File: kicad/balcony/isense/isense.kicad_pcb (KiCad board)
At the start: 2 copper layers, 20.3 x 15.2 mm, 9 parts, among them J1 IN, U1 OPA237NA_250, U2 OPA237NA_250

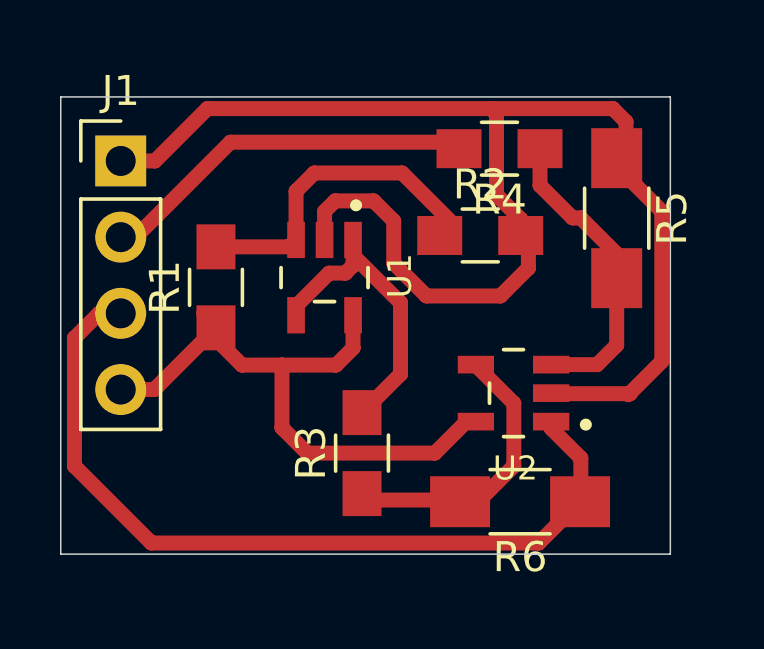
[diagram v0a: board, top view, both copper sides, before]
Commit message: Various schematic fixes
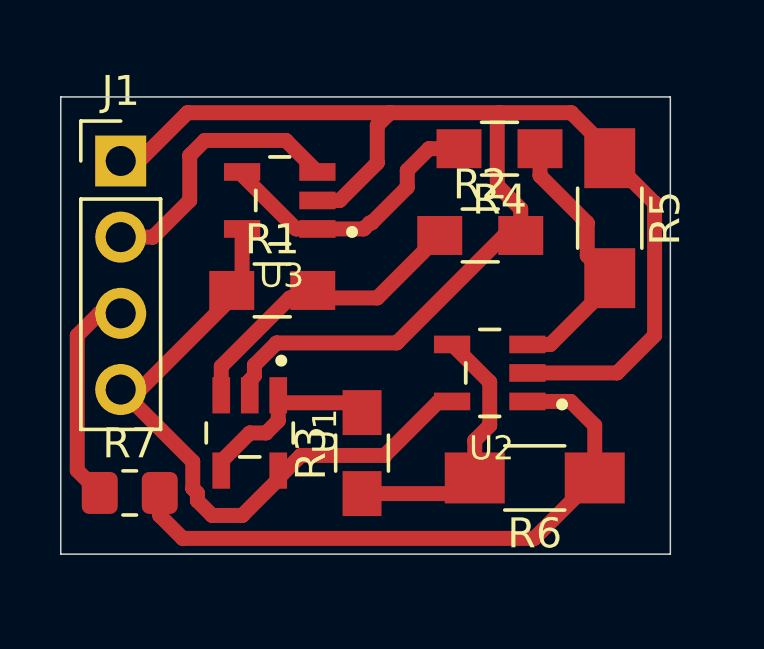
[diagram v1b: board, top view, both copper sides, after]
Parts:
- added R7: 100K, Resistor_SMD:R_0805_2012Metric_Pad1.20x1.40mm_HandSolder, F.Cu at (78.5, 64.0)
- added U3: OPA237NA_250, OPA237NA:SOT95P280X145-5N, F.Cu at (83.5, 54.2)
- moved U1 5.75 mm to (82.5, 62.0)
- moved R1 1.88 mm to (83.2, 57.2), turned to 0 degrees
- moved U2 1.04 mm to (90.5, 60.0)
- moved R6 0.93 mm to (92.0, 63.5)
- moved R5 0.23 mm to (94.5, 54.8)
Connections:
- R4 pad 2: /VIN -> Net-(R4-Pad2)
- R6 pad 1: /VOUT -> Net-(R6-Pad1)
- U2 pad 1: /VOUT -> Net-(R6-Pad1)
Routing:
- net /VOUT: track 28.3 -> 7.31 mm
- net Net-(R6-Pad1): track 0.00 -> 20.7 mm
- net Net-(R4-Pad2): track 0.00 -> 9.51 mm
- net Net-(R3-Pad2): track 10.6 -> 6.54 mm
- net /VIN: track 12.7 -> 9.20 mm
- net GND: track 46.2 -> 49.4 mm
- net +5V: track 20.7 -> 22.5 mm
- net Net-(R4-Pad1): track 10.2 -> 9.17 mm
